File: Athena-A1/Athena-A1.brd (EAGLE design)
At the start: 33 x 59.6 mm, 86 parts, among them J1 MF-CON-MICROUSB-RIGHT, J2 TC2030-IDC-NL, J3 MF-CON-2.54mm-01x08, J4 MF-CON-2.54mm-01x08, J5 MF-CON-2.54mm-01x07, SW1 MF-SW-TACT-6MM, SW2 MF-SW-TACT-6MM, U1 PRTR5V0U2X,215, U2 MCP73831T-2ACI/OT, U3 AP2112K-3.3TRG1, U4 RT9080-18GJ5, U5 MK22FN128VLH10, U6 FE310, U7 32MBit, X1 JST 2-Pin, X2 MIKROE_CLICKMINI, Y1 TSX-3225-16.0000MF18X-AC0, Y2 KX3211A0032.768000

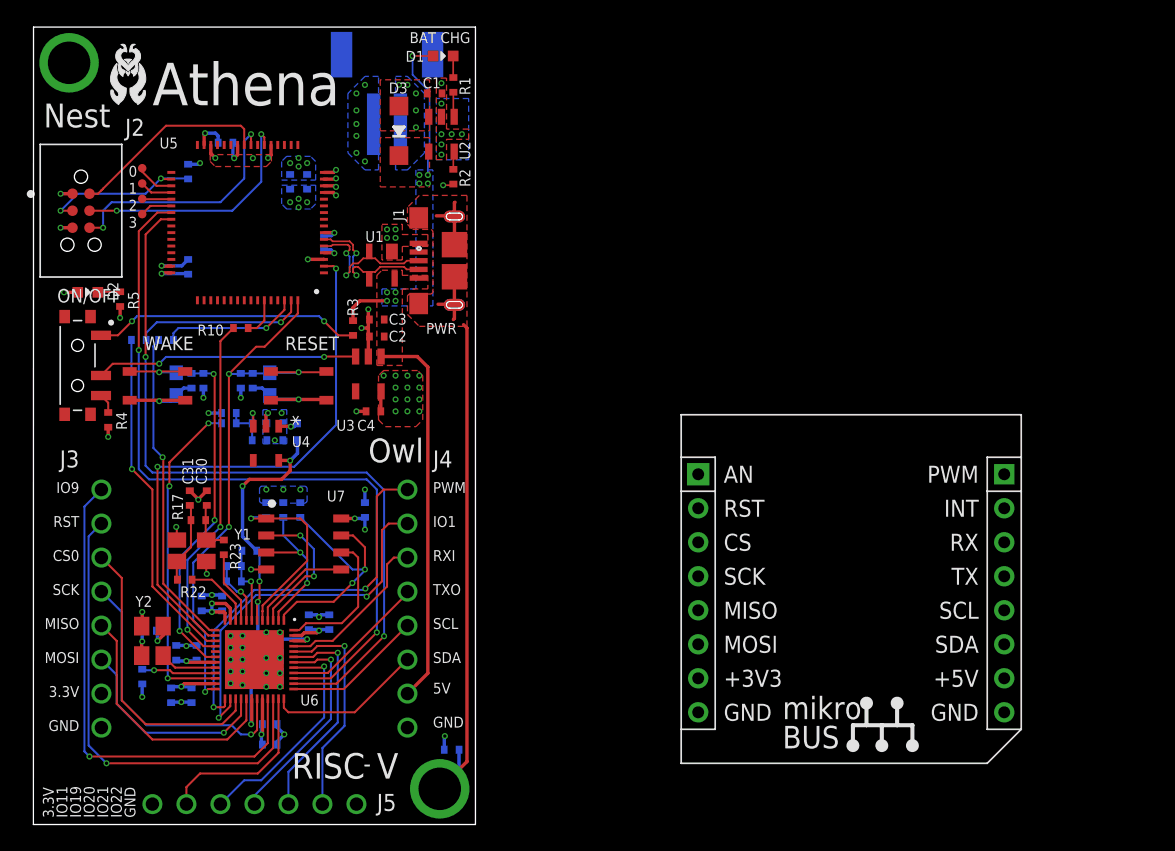
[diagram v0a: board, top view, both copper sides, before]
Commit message: Finished updates post-review
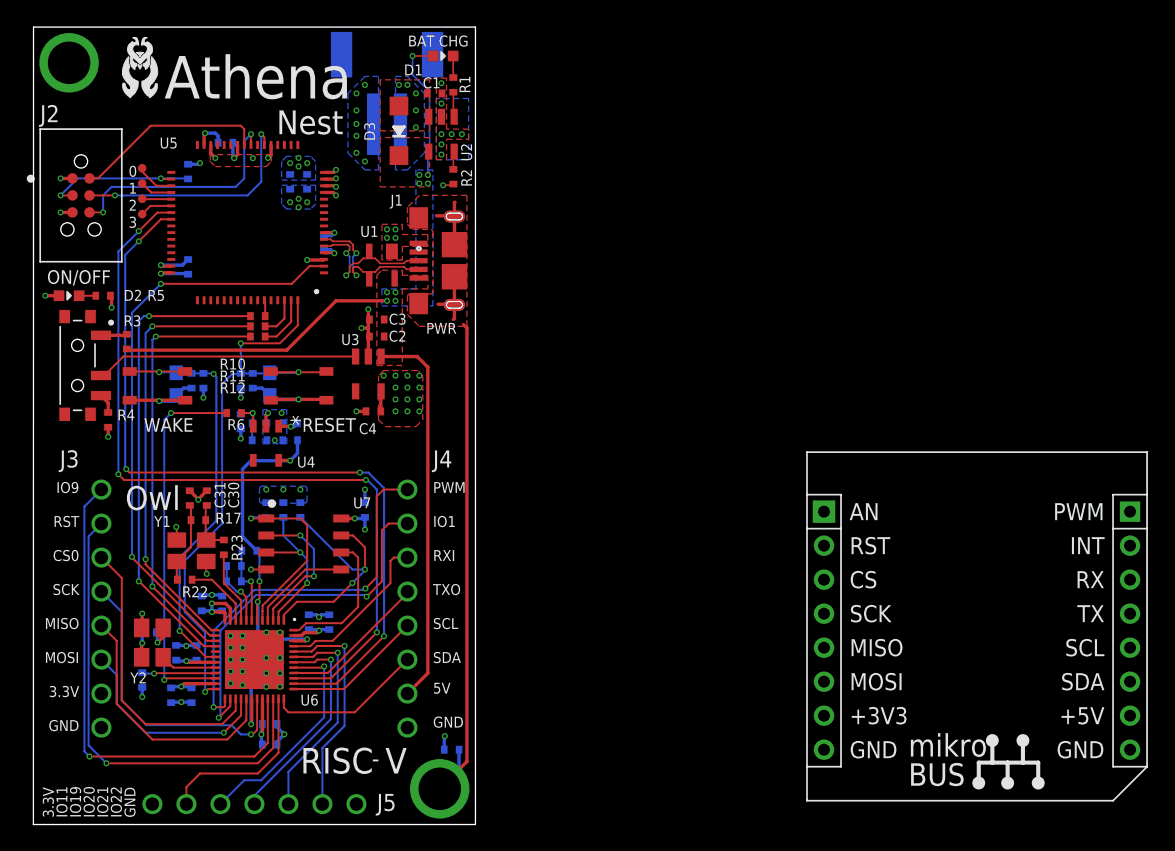
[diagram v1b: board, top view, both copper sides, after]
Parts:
- moved R3 16.9 mm to (6.99, 36.1), turned to 270 degrees
- moved X2 9.80 mm to (57.8, 1.78)
- moved R12 8.89 mm to (16.8, 36.4), flipped to the top, turned to 0 degrees
- moved R11 6.93 mm to (16.8, 37.2), flipped to the top, turned to 180 degrees
- moved R10 1.55 mm to (16.8, 38.0)
- moved D2 1.42 mm to (2.67, 39.5)
- moved R5 1.30 mm to (5.21, 39.5), turned to 0 degrees
- moved J2 1.14 mm to (3.56, 47.0)
- moved R7 1.09 mm to (15.5, 30.1), turned to 270 degrees
- moved R6 0.85 mm to (15.0, 30.7), flipped to the top, turned to 0 degrees
- moved R15 0.25 mm to (8.13, 10.8)
- moved C32 0.13 mm to (8.64, 14.4)
- moved Y2 0.13 mm to (8.89, 13.6)
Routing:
- net N$1: track 20.0 -> 1.95 mm, vias 2 -> 0
- net V_USB: track 43.6 -> 60.8 mm
- net JTAG_TDI: track 26.6 -> 35.6 mm
- net N$8: track 12.9 -> 4.01 mm, vias 1 -> 0
- net JTAG_TCK: track 24.0 -> 32.6 mm, vias 1 -> 2
- net N$9: track 10.2 -> 3.04 mm, vias 1 -> 0
- net JTAG_TMS: track 25.4 -> 32.2 mm, vias 1 -> 2
- net VDD_CORE_EN: track 24.8 -> 28.2 mm, vias 3 -> 2
- net UART_RX_MK22: track 57.5 -> 59.9 mm, vias 2 -> 4
- net UART_TX_MK22: track 57.4 -> 59.7 mm, vias 2 -> 4
- net N$11: track 2.95 -> 1.21 mm
- net RESET: track 43.5 -> 44.8 mm, vias 4 -> 3
- net JTAG_TDO: track 42.0 -> 42.7 mm
- net 1.8V: track 34.2 -> 34.5 mm, vias 6 -> 5
- net WAKE: track 32.1 -> 32.2 mm, vias 4 -> 3
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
